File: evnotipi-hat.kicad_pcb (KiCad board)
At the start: 2 copper layers, 65 x 30.5 mm, 6 parts, among them J1 RPi_GPIO, J2 RPi_GPIO

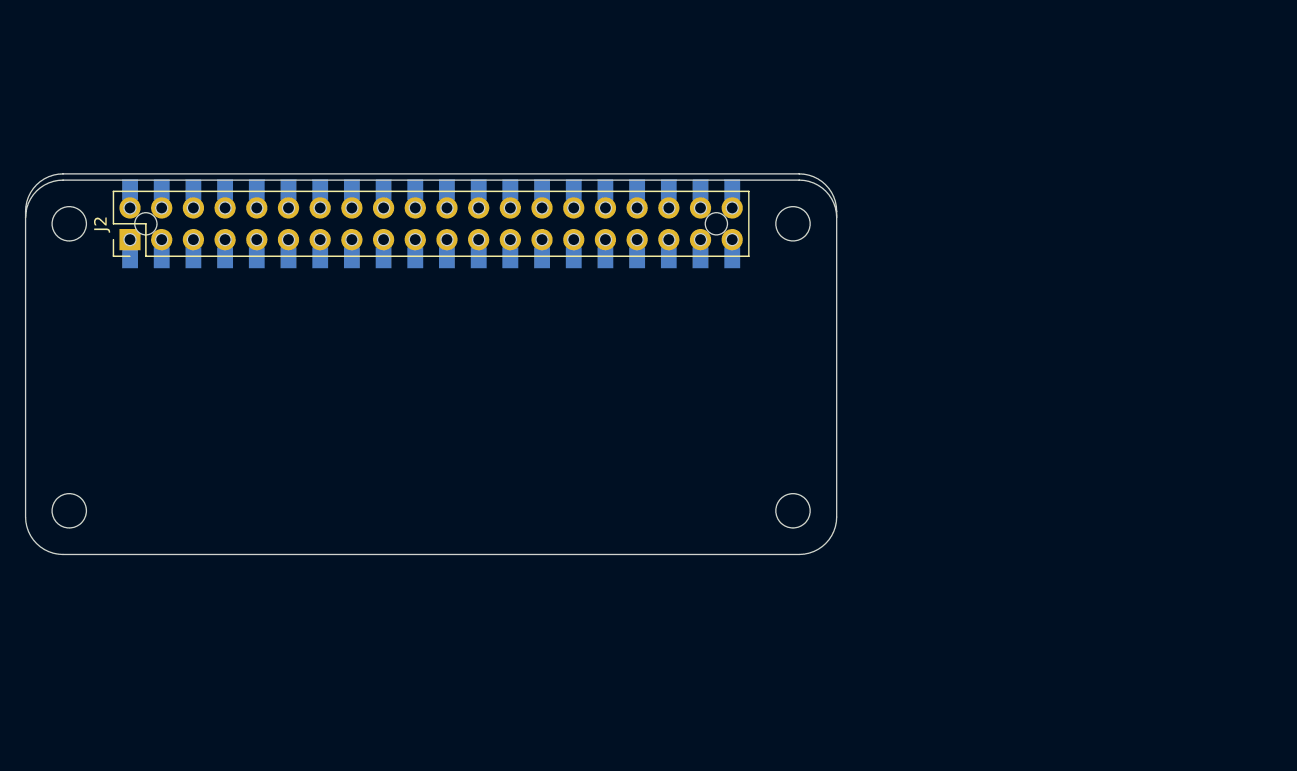
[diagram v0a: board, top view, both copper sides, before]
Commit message: Redesigned again. Prototype 1
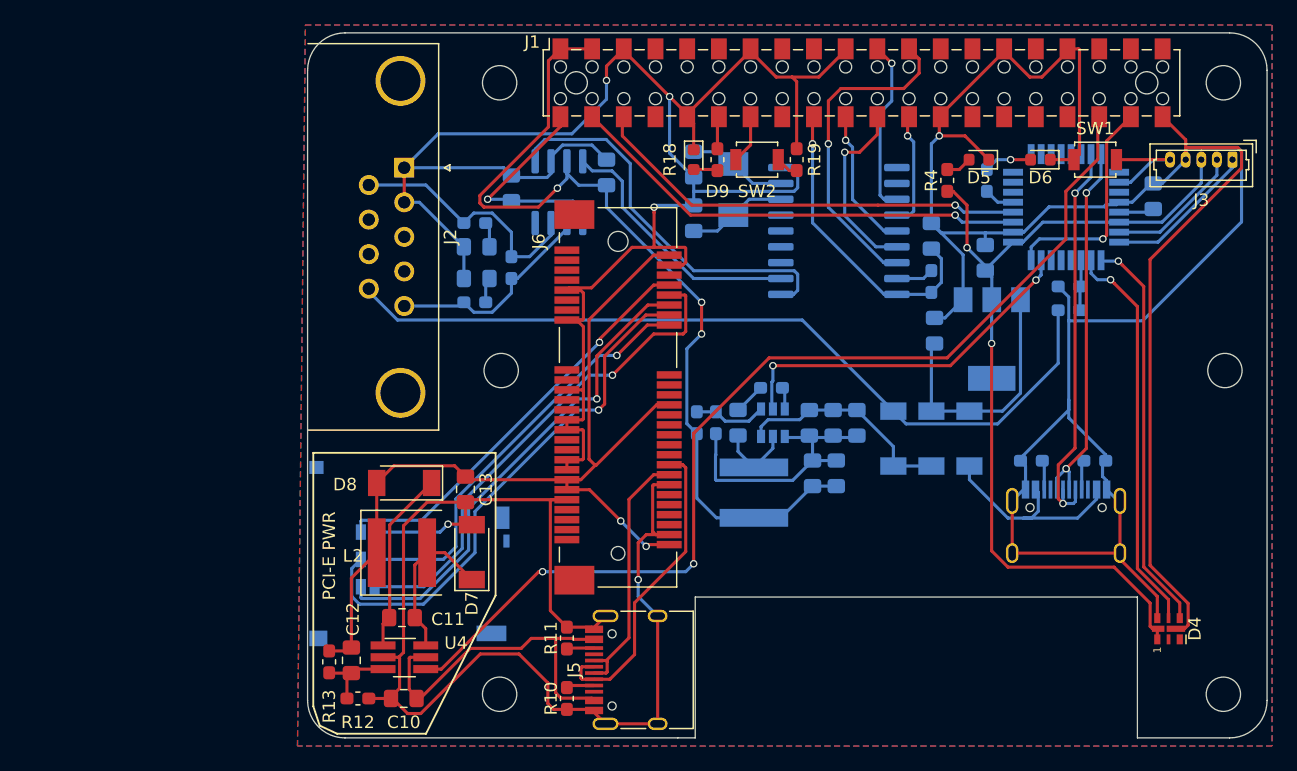
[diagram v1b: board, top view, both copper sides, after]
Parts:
- removed the ? at (16.0, 51.0)
- added ?: , RPi_Hat:RPi_Hat_Mounting_Hole, F.Cu at (108.6, 39.8)
- added ?: , RPi_Hat:RPi_Hat_Mounting_Hole, F.Cu at (50.6, 39.8)
- added ?: , RPi_Hat:RPi_Hat_Mounting_Hole, F.Cu at (50.5, 65.7)
- added C1: 10µF, Capacitor_SMD:C_0805_2012Metric_Pad1.15x1.40mm_HandSolder, B.Cu at (79.1, 44.0)
- added C10: 10µF, Capacitor_SMD:C_0805_2012Metric_Pad1.15x1.40mm_HandSolder, F.Cu at (42.8, 66.0)
- added C11: 0.01µF, Capacitor_SMD:C_0805_2012Metric_Pad1.15x1.40mm_HandSolder, F.Cu at (42.7, 59.6)
- added C12: 1000pF, Capacitor_SMD:C_0805_2012Metric_Pad1.15x1.40mm_HandSolder, F.Cu at (38.6, 63.0)
- added C13: 22µF, Capacitor_SMD:C_0805_2012Metric_Pad1.15x1.40mm_HandSolder, F.Cu at (47.8, 49.3)
- added C14: 22pF, Capacitor_SMD:C_0805_2012Metric_Pad1.15x1.40mm_HandSolder, B.Cu at (66.0, 27.6)
- added C15: 22pF, Capacitor_SMD:C_0805_2012Metric_Pad1.15x1.40mm_HandSolder, B.Cu at (66.0, 23.2)
- added C16: 100nF, Capacitor_SMD:C_0805_2012Metric_Pad1.15x1.40mm_HandSolder, B.Cu at (85.1, 29.0)
- added C17: 100nF, Capacitor_SMD:C_0805_2012Metric_Pad1.15x1.40mm_HandSolder, B.Cu at (51.4, 25.2)
- added C18: 100nF, Capacitor_SMD:C_0805_2012Metric_Pad1.15x1.40mm_HandSolder, B.Cu at (59.1, 23.9)
- added C19: 560pF, Capacitor_SMD:C_0805_2012Metric_Pad1.15x1.40mm_HandSolder, B.Cu at (48.6, 32.4)
- added C2: 10µF, Capacitor_SMD:C_0805_2012Metric_Pad1.15x1.40mm_HandSolder, B.Cu at (77.2, 44.0)
- added C20: 560pF, Capacitor_SMD:C_0805_2012Metric_Pad1.15x1.40mm_HandSolder, B.Cu at (48.6, 29.8)
- added C3: 100nF, Capacitor_SMD:C_0805_2012Metric_Pad1.15x1.40mm_HandSolder, B.Cu at (75.3, 44.0)
- added C4: 100nF, Capacitor_SMD:C_0805_2012Metric_Pad1.15x1.40mm_HandSolder, B.Cu at (69.6, 43.9)
- added C5: 22µF, Capacitor_SMD:C_0805_2012Metric_Pad1.15x1.40mm_HandSolder, B.Cu at (77.5, 48.0)
- added C6: 22µF, Capacitor_SMD:C_0805_2012Metric_Pad1.15x1.40mm_HandSolder, B.Cu at (75.6, 48.0)
- added C7: 10µF, Capacitor_SMD:C_0805_2012Metric_Pad1.15x1.40mm_HandSolder, B.Cu at (85.3, 36.6)
- added C8: 22µF, Capacitor_SMD:C_0805_2012Metric_Pad1.15x1.40mm_HandSolder, B.Cu at (89.4, 30.7)
- added C9: 1µF, Capacitor_SMD:C_0805_2012Metric_Pad1.15x1.40mm_HandSolder, B.Cu at (102.9, 25.8)
- added D1: D_Schottky, Diode_SMD:D_SOD-128, B.Cu at (82.0, 45.2)
- added D2: D_Schottky, Diode_SMD:D_SOD-128, B.Cu at (88.1, 45.2)
- added D3: D_Schottky, Diode_SMD:D_SOD-128, B.Cu at (85.1, 45.2)
- added D4: APA102-2020, LED_SMD:LED-APA102-2020, F.Cu at (104.1, 60.5)
- added D5: green, LED_SMD:LED_0603_1608Metric, F.Cu at (88.9, 22.9)
- added D6: red, LED_SMD:LED_0603_1608Metric, F.Cu at (93.8, 22.9)
- added D7: D_Schottky 1A, Diode_SMD:D_SOD-128, F.Cu at (48.3, 54.3)
- added D8: 1N4148W, Diode_SMD:D_SOD-128, F.Cu at (42.8, 48.8)
- added D9: blue, LED_SMD:LED_0603_1608Metric, F.Cu at (66.0, 22.9)
- added J3: Conn_01x05_Male, Connector_Molex:Molex_PicoBlade_53047-0510_1x05_P1.25mm_Vertical, F.Cu at (109.2, 22.9)
- added J4: USB_C_Receptacle_USB2.0, Connector_USB:USB_C_Receptacle_HRO_TYPE-C-31-M-12, B.Cu at (95.9, 53.3)
- added J5: USB_C_Receptacle_USB2.0, Connector_USB:USB_C_Receptacle_HRO_TYPE-C-31-M-12, F.Cu at (62.1, 63.8)
- added J6: Bus_PCI_Express_Mini, Connector_PCBEdge:BUS_PCI_Express_Mini_Full, F.Cu at (60.0, 41.9)
- added J7: SIM_Card, Connector_JAE_mine:SF56S006V4BR2000, B.Cu at (39.4, 52.7)
- added L1: 5,6µH, Inductor_SMD:L_Coilcraft_XAL60xx_6.36x6.56mm, B.Cu at (70.9, 49.5)
- added L2: 4,7µH, Inductor_SMD:L_Coilcraft_XAL60xx_6.36x6.56mm, F.Cu at (42.7, 54.4)
- added R1: R10k, Resistor_SMD:R_0603_1608Metric_Pad1.05x0.95mm_HandSolder, B.Cu at (67.8, 43.9)
- added R10: 5K1, Resistor_SMD:R_0603_1608Metric_Pad1.05x0.95mm_HandSolder, F.Cu at (55.9, 66.0)
- added R11: 5K1, Resistor_SMD:R_0603_1608Metric_Pad1.05x0.95mm_HandSolder, F.Cu at (55.9, 61.2)
- added R12: 10k, Resistor_SMD:R_0603_1608Metric_Pad1.05x0.95mm_HandSolder, F.Cu at (39.1, 66.0)
- added R13: 31,6k, Resistor_SMD:R_0603_1608Metric_Pad1.05x0.95mm_HandSolder, F.Cu at (36.8, 63.1)
- added R14: 4k7, Resistor_SMD:R_0603_1608Metric_Pad1.05x0.95mm_HandSolder, B.Cu at (85.1, 32.6)
- added R15: R120, Resistor_SMD:R_0603_1608Metric_Pad1.05x0.95mm_HandSolder, B.Cu at (51.4, 31.5)
- added R16: 100R, Resistor_SMD:R_0603_1608Metric_Pad1.05x0.95mm_HandSolder, B.Cu at (48.5, 34.3)
- added R17: 100R, Resistor_SMD:R_0603_1608Metric_Pad1.05x0.95mm_HandSolder, B.Cu at (48.5, 27.9)
- added R18: R15, Resistor_SMD:R_0603_1608Metric_Pad1.05x0.95mm_HandSolder, F.Cu at (67.9, 22.9)
- added R19: 10K, Resistor_SMD:R_0603_1608Metric_Pad1.05x0.95mm_HandSolder, F.Cu at (74.3, 22.9)
- added R2: 30R, Resistor_SMD:R_0603_1608Metric_Pad1.05x0.95mm_HandSolder, B.Cu at (72.3, 41.1)
- added R3: 52,3k, Resistor_SMD:R_0603_1608Metric_Pad1.05x0.95mm_HandSolder, B.Cu at (66.3, 43.9)
- added R4: 10K, Resistor_SMD:R_0603_1608Metric_Pad1.05x0.95mm_HandSolder, F.Cu at (86.4, 24.5)
- added R5: 5K1, Resistor_SMD:R_0603_1608Metric_Pad1.05x0.95mm_HandSolder, B.Cu at (98.2, 47.0)
- added R6: 5K1, Resistor_SMD:R_0603_1608Metric_Pad1.05x0.95mm_HandSolder, B.Cu at (93.1, 47.0)
- added R7: 100K, Resistor_SMD:R_0603_1608Metric_Pad1.05x0.95mm_HandSolder, B.Cu at (96.1, 34.9)
- added R8: 27K, Resistor_SMD:R_0603_1608Metric_Pad1.05x0.95mm_HandSolder, B.Cu at (96.1, 33.0)
- added R9: 1.5K, Resistor_SMD:R_0603_1608Metric_Pad1.05x0.95mm_HandSolder, B.Cu at (89.5, 24.5)
- added SW1: SW_Reset, Button_Switch_SMD:SW_SPST_B3U-1000P, F.Cu at (98.2, 22.9)
- added SW2: SW_Reset, Button_Switch_SMD:SW_SPST_B3U-1000P, F.Cu at (71.1, 22.9)
- added U1: TPS56339DDC, Package_TO_SOT_SMD:SOT-23-6, B.Cu at (72.4, 43.9)
- added U2: AZ1117-3.3, Package_TO_SOT_SMD:SOT-223, B.Cu at (89.9, 37.2)
- added U3: ATSAMD21E18A-A, Package_QFP:TQFP-32_7x7mm_P0.8mm, B.Cu at (95.9, 26.7)
- added U4: LM2734Y, Package_TO_SOT_SMD:TSOT-23-6_HandSoldering, F.Cu at (42.9, 62.7)
- added U5: MCP2515-xSO, Package_SO:SOIC-18W_7.5x11.6mm_P1.27mm, B.Cu at (77.7, 28.6)
- added U6: MCP2562-E-SN, Package_SO:SOIC-8_3.9x4.9mm_P1.27mm, B.Cu at (55.2, 25.5)
- added Y1: 16MHz, Crystal:Crystal_SMD_Abracon_ABM3-2Pin_5.0x3.2mm, B.Cu at (69.2, 25.3)
- J1: footprint Connector_Samtec_HLE_SMD-ML:Samtec_HLE-120-02-xxx-DV-BE-A_2x20_RPi_Bottom -> Connector_Samtec_HLE_SMD-ML:Samtec_HLE-120-02-xxx-DV-BE-A_2x20_RPi_Top; moved to F.Cu
- J2: value RPi_GPIO -> DB9_Male_MountingHoles; footprint Connector_PinHeader_2.54mm:PinHeader_2x20_P2.54mm_Vertical -> Connector_Dsub:DSUB-9_Male_Horizontal_P2.77x2.84mm_EdgePinOffset4.94mm_Housed_MountingHolesOffset7.48mm
- moved ? 37.5 mm to (108.5, 65.7)
- moved ? 36.3 mm to (50.5, 16.7)
- moved ? 36.3 mm to (108.5, 16.7)
- moved J1 36.3 mm to (79.5, 16.7)
- moved J2 22.7 mm to (42.8, 23.5), turned to 270 degrees
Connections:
- J1 pad 1: Net-(J1-Pad1) -> +3V3
- J1 pad 10: Net-(J1-Pad10) -> (no net)
- J1 pad 11: Net-(J1-Pad11) -> RPI_LED
- J1 pad 12: Net-(J1-Pad12) -> (no net)
- J1 pad 13: Net-(J1-Pad13) -> RPI_CMD
- J1 pad 14: Net-(J1-Pad14) -> GND
- J1 pad 15: Net-(J1-Pad15) -> (no net)
- J1 pad 16: Net-(J1-Pad16) -> (no net)
- J1 pad 17: Net-(J1-Pad17) -> +3V3
- J1 pad 18: Net-(J1-Pad18) -> (no net)
- J1 pad 19: Net-(J1-Pad19) -> MOSI
- J1 pad 2: Net-(J1-Pad2) -> +5V
- J1 pad 20: Net-(J1-Pad20) -> GND
- J1 pad 21: Net-(J1-Pad21) -> MISO
- J1 pad 22: Net-(J1-Pad22) -> RXINT
- J1 pad 23: Net-(J1-Pad23) -> SPI_CLK
- J1 pad 24: Net-(J1-Pad24) -> SPI_CE0
- J1 pad 25: Net-(J1-Pad25) -> GND
- J1 pad 26: Net-(J1-Pad26) -> (no net)
- J1 pad 27: Net-(J1-Pad27) -> (no net)
- J1 pad 28: Net-(J1-Pad28) -> (no net)
- J1 pad 29: Net-(J1-Pad29) -> (no net)
- J1 pad 3: Net-(J1-Pad3) -> SDA
- J1 pad 30: Net-(J1-Pad30) -> GND
- J1 pad 31: Net-(J1-Pad31) -> (no net)
- J1 pad 32: Net-(J1-Pad32) -> (no net)
- J1 pad 33: Net-(J1-Pad33) -> (no net)
- J1 pad 34: Net-(J1-Pad34) -> GND
- J1 pad 35: Net-(J1-Pad35) -> PCIE_PWR_EN
- J1 pad 36: Net-(J1-Pad36) -> (no net)
- J1 pad 37: Net-(J1-Pad37) -> Pi_Running
- J1 pad 38: Net-(J1-Pad38) -> (no net)
- J1 pad 39: Net-(J1-Pad39) -> GND
- J1 pad 4: Net-(J1-Pad4) -> +5V
- J1 pad 40: Net-(J1-Pad40) -> (no net)
- J1 pad 5: Net-(J1-Pad5) -> SCL
- J1 pad 6: Net-(J1-Pad6) -> GND
- J1 pad 7: Net-(J1-Pad7) -> (no net)
- J1 pad 8: Net-(J1-Pad8) -> (no net)
- J1 pad 9: Net-(J1-Pad9) -> GND
- J2 pad 1: Net-(J2-Pad1) -> GND
- J2 pad 2: Net-(J2-Pad2) -> GND
- J2 pad 3: Net-(J2-Pad3) -> (no net)
- J2 pad 4: Net-(J2-Pad4) -> (no net)
- J2 pad 5: Net-(J2-Pad5) -> CAN_L
- J2 pad 6: Net-(J2-Pad6) -> CAN_H
- J2 pad 7: Net-(J2-Pad7) -> (no net)
- J2 pad 8: Net-(J2-Pad8) -> (no net)
- J2 pad 9: Net-(J2-Pad9) -> +12P
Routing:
- net GND: track 0.00 -> 490.1 mm, vias 0 -> 6
- net PCIE_PWR_EN: track 0.00 -> 83.2 mm, vias 0 -> 2
- net +3.3VA: track 0.00 -> 74.3 mm, vias 0 -> 2
- net +5V: track 0.00 -> 73.5 mm, vias 0 -> 3
- net +3.3VP: track 0.00 -> 70.6 mm, vias 0 -> 2
- net +12P: track 0.00 -> 66.1 mm
- net Net-(J6-Pad14): track 0.00 -> 42.7 mm, vias 0 -> 1
- net +3V3: track 0.00 -> 42.7 mm, vias 0 -> 2
- net Net-(J6-Pad10): track 0.00 -> 39.8 mm, vias 0 -> 1
- net Net-(J6-Pad12): track 0.00 -> 39.3 mm, vias 0 -> 1
- net SDA: track 0.00 -> 37.2 mm, vias 0 -> 1
- net SCL: track 0.00 -> 35.4 mm, vias 0 -> 1
- net Net-(J6-Pad16): track 0.00 -> 33.6 mm, vias 0 -> 1
- net Net-(J6-Pad8): track 0.00 -> 33.6 mm, vias 0 -> 1
- net /Watchdog/USB_D-: track 0.00 -> 32.4 mm, vias 0 -> 2
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- added copper zone on B.Cu, net GND
- added copper zone on F.Cu, net GND
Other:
- board size 65 x 30.5 mm -> 76.9 x 56.5 mm
- board text added: "CAN If"
- board text added: "Main 5V Pwr"
- board text added: "PCI-E PWR"
- board text added: "W.Dog Pwr"
- board text added: "Watchdog"
- board text removed: "Select one of these board edges depending upon the type of socket that is used."
